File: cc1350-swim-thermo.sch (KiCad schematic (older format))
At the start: 54 parts, among them P1 LMT_70_1, P2 LMT_70_2, P3 SMA FEMALE, P4 USB_OTG, P5 CONN_02X05, Q1 2N7002, SW1 SW_Push, U1 2450BM14G0011T, U2 XMSSJE3G0PA-003, U3 CC1350F128RSM, U4 TLV713, U5 TLC5973, U6 MCP16251, U7 LFB18868MBG9E212, Y1 24MHz, Y2 32.768kHz

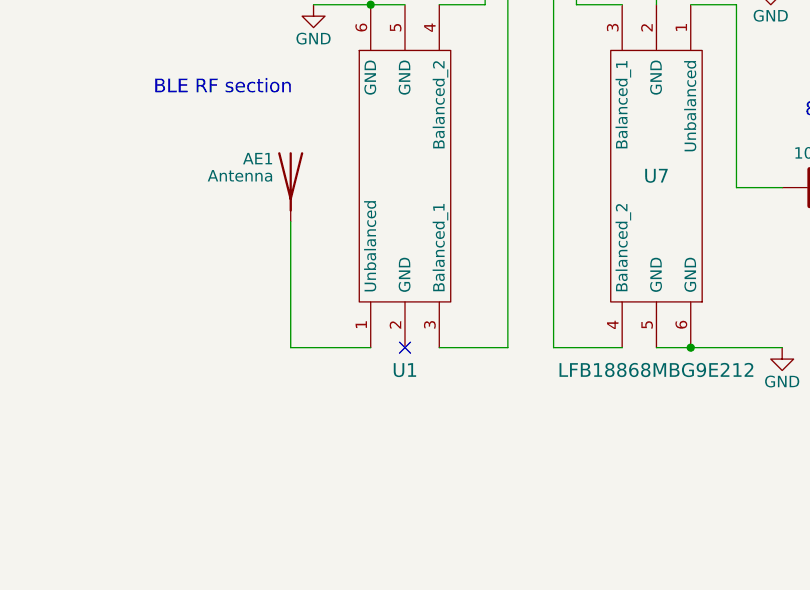
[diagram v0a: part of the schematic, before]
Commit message: started wiring
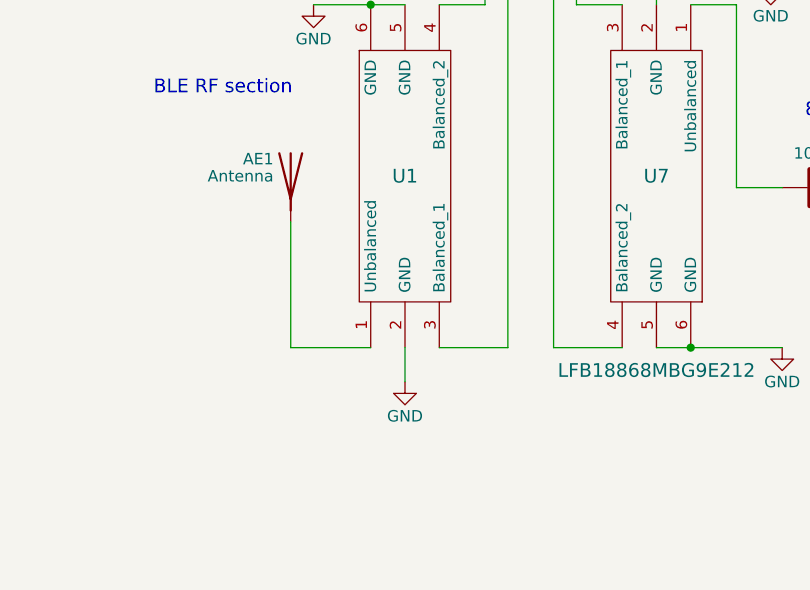
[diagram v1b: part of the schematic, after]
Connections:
- net GND: now also U1.2 (GND)
- no-connect marks 8 -> 7
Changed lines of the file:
@@
 U 1 1 58C40E34
 P 3350 6650
-F 0 "U1" H 3350 7500 60  0000 C CNN
+F 0 "U1" H 3350 6650 60  0000 C CNN
 F 1 "2450BM14G0011T" H 3350 5800 60  0000 C CNN
 F 2 "cc1350:2450BM14G011T" H 3150 6650 60  0001 C CNN
@@
 	1    0    0    -1
 $EndComp
-NoConn ~ 3350 7400
 NoConn ~ 5300 12700
 $Comp
@@
 Wire Wire Line
 	4800 6700 5000 6700
+$Comp
+L GND #PWR?
+U 1 1 58D96477
+P 3350 7550
+F 0 "#PWR?" H 3350 7300 50  0001 C CNN
+F 1 "GND" H 3350 7400 50  0000 C CNN
+F 2 "" H 3350 7550 50  0000 C CNN
+F 3 "" H 3350 7550 50  0000 C CNN
+	1    3350 7550
+	1    0    0    -1
+$EndComp
+Wire Wire Line
+	3350 7400 3350 7550
 $EndSCHEMATC
